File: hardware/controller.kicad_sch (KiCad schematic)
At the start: 5 parts, among them Q1 BC848

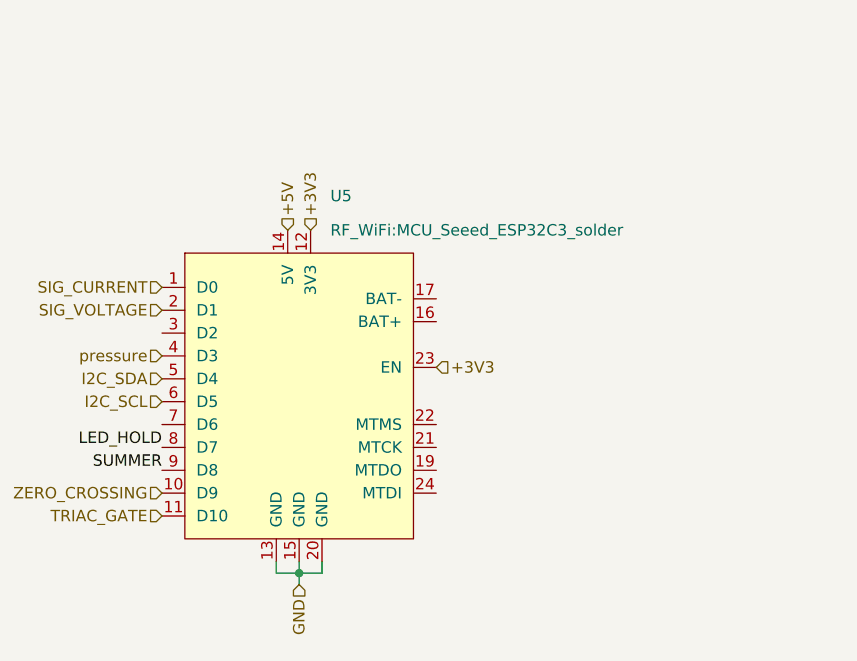
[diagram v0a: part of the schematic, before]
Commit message: done routing
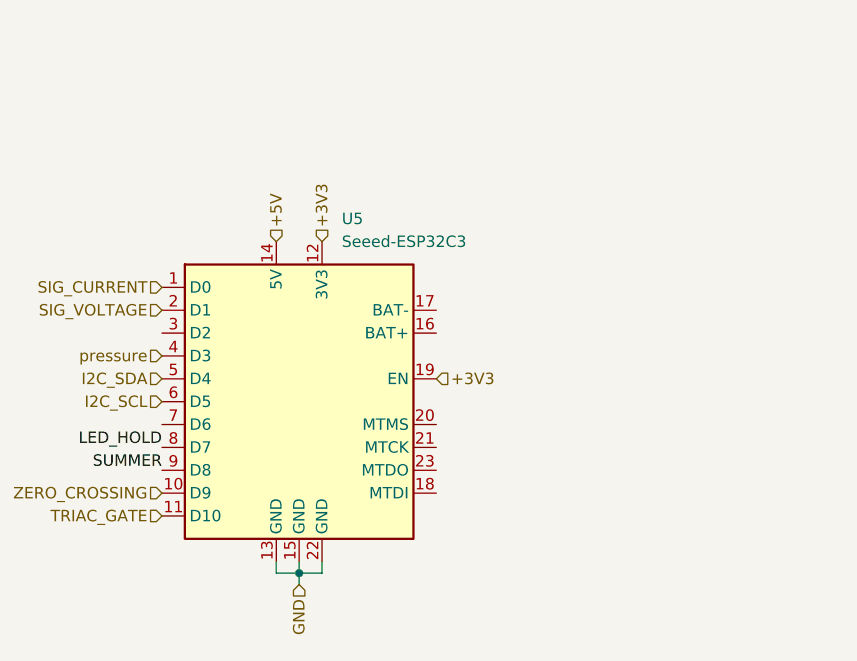
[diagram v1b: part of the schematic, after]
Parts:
- U5: value ~ -> Seeed-ESP32C3; footprint RF_WiFi:MCU_Seeed_ESP32C3_solder -> RF_Module:MCU_Seeed_ESP32C3_HandSolder
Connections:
- net +3V3: now also U5.19 (EN); no longer U5.23 (EN)
- net GND: now also U5.22 (GND); no longer U5.20 (GND)
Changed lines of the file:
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@@
 	(hierarchical_label "+3V3"
 		(shape input)
-		(at 147.32 85.09 0)
+		(at 147.32 86.36 0)
 		(fields_autoplaced yes)
 		(effects
@@
 	(hierarchical_label "+3V3"
 		(shape input)
-		(at 133.35 69.85 90)
+		(at 134.62 71.12 90)
 		(fields_autoplaced yes)
 		(effects
@@
 	(hierarchical_label "+5V"
 		(shape input)
-		(at 130.81 69.85 90)
+		(at 129.54 71.12 90)
 		(fields_autoplaced yes)
 		(effects
@@
 				(path "/ae153005-c1c4-4678-92de-98a47cf88e8d/421ee7c4-2a9c-4e65-b00b-3d6ff22b5783"
 					(reference "BZ1")
-					(unit 1)
-				)
-			)
-		)
-	)
-	(symbol
-		(lib_id "MCU_Seeed_ESP32C3:Seeed-ESP32C3")
-		(at 132.08 85.09 0)
-		(unit 1)
-		(exclude_from_sim no)
-		(in_bom yes)
-		(on_board yes)
-		(dnp no)
-		(fields_autoplaced yes)
-		(property "Reference" "U5"
-			(at 135.5441 66.04 0)
-			(effects
-				(font
-					(size 1.27 1.27)
-				)
-				(justify left)
-			)
-		)
-		(property "Value" "~"
-			(at 135.5441 68.58 0)
-			(effects
-				(font
-					(size 1.27 1.27)
-				)
-				(justify left)
-			)
-		)
-		(property "Footprint" "RF_WiFi:MCU_Seeed_ESP32C3_solder"
-			(at 135.5441 69.85 0)
-			(effects
-				(font
-					(size 1.27 1.27)
-				)
-				(justify left)
-			)
-		)
-		(property "Datasheet" ""
-			(at 132.08 85.09 0)
-			(effects
-				(font
-					(size 1.27 1.27)
-				)
-				(hide yes)
-			)
-		)
-		(property "Description" ""
-			(at 132.08 85.09 0)
-			(effects
-				(font
-					(size 1.27 1.27)
-				)
-				(hide yes)
-			)
-		)
-		(pin "6"
-		)
-		(pin "11"
-		)
-		(pin "14"
-		)
-		(pin "21"
-		)
-		(pin "13"
-		)
-		(pin "10"
-		)
-		(pin "12"
-		)
-		(pin "1"
-		)
-		(pin "20"
-		)
-		(pin "22"
-		)
-		(pin "24"
-		)
-		(pin "5"
-		)
-		(pin "23"
-		)
-		(pin "9"
-		)
-		(pin "19"
-		)
-		(pin "4"
-		)
-		(pin "8"
-		)
-		(pin "7"
-		)
-		(pin "2"
-		)
-		(pin "17"
-		)
-		(pin "15"
-		)
-		(pin "16"
-		)
-		(pin "3"
-		)
-		(instances
-			(project "Steuerplatine"
-				(path "/ae153005-c1c4-4678-92de-98a47cf88e8d/421ee7c4-2a9c-4e65-b00b-3d6ff22b5783"
-					(reference "U5")
 					(unit 1)
 				)
@@
 					(unit 1)
 				)
+			)
+		)
+	)
+	(symbol
+		(lib_name "Seeed-ESP32C3_1")
+		(lib_id "MCU_Seeed_ESP32C3:Seeed-ESP32C3")
+		(at 132.08 88.9 0)
+		(unit 1)
+		(exclude_from_sim no)
+		(in_bom yes)
+		(on_board yes)
+		(dnp no)
+		(fields_autoplaced yes)
+		(property "Reference" "U5"
+			(at 136.8141 68.58 0)
+			(effects
+				(font
+					(size 1.27 1.27)
+				)
+				(justify left)
+			)
+		)
+		(property "Value" "Seeed-ESP32C3"
+			(at 136.8141 71.12 0)
+			(effects
+				(font
+					(size 1.27 1.27)
+				)
+				(justify left)
+			)
+		)
+		(property "Footprint" "RF_Module:MCU_Seeed_ESP32C3_HandSolder"
+			(at 132.842 117.094 0)
+			(effects
+				(font
+					(size 1.27 1.27)
+				)
+				(hide yes)
+			)
+		)
+		(property "Datasheet" "https://wiki.seeedstudio.com/XIAO_ESP32C3_Getting_Started/"
+			(at 132.588 119.126 0)
+			(effects
+				(font
+					(size 1.27 1.27)
+				)
+				(hide yes)
+			)
+		)
+		(property "Description" "Wifi Module based on ESP32C3"
+			(at 132.08 85.09 0)
+			(effects
+				(font
+					(size 1.27 1.27)
+				)
+				(hide yes)
+			)
+		)
+		(pin "8"
+		)
+		(pin "14"
+		)
+		(pin "18"
+		)
+		(pin "17"
+		)
+		(pin "3"
+		)
+		(pin "10"
+		)
+		(pin "13"
+		)
+		(pin "12"
+		)
+		(pin "11"
+		)
+		(pin "1"
+		)
+		(pin "6"
+		)
+		(pin "7"
+		)
+		(pin "4"
+		)
+		(pin "21"
+		)
+		(pin "20"
+		)
+		(pin "19"
+		)
+		(pin "2"
+		)
+		(pin "23"
+		)
+		(pin "16"
+		)
+		(pin "5"
+		)
+		(pin "9"
+		)
+		(pin "22"
+		)
+		(pin "15"
+		)
+		(instances
+			(project "Steuerplatine"
+				(path "/ae153005-c1c4-4678-92de-98a47cf88e8d/421ee7c4-2a9c-4e65-b00b-3d6ff22b5783"
+					(reference "U5")
+					(unit 1)
+				)
